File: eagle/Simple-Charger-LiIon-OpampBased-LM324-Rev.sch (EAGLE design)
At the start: 21 parts, among them IC1 LM324N, T1 BC327

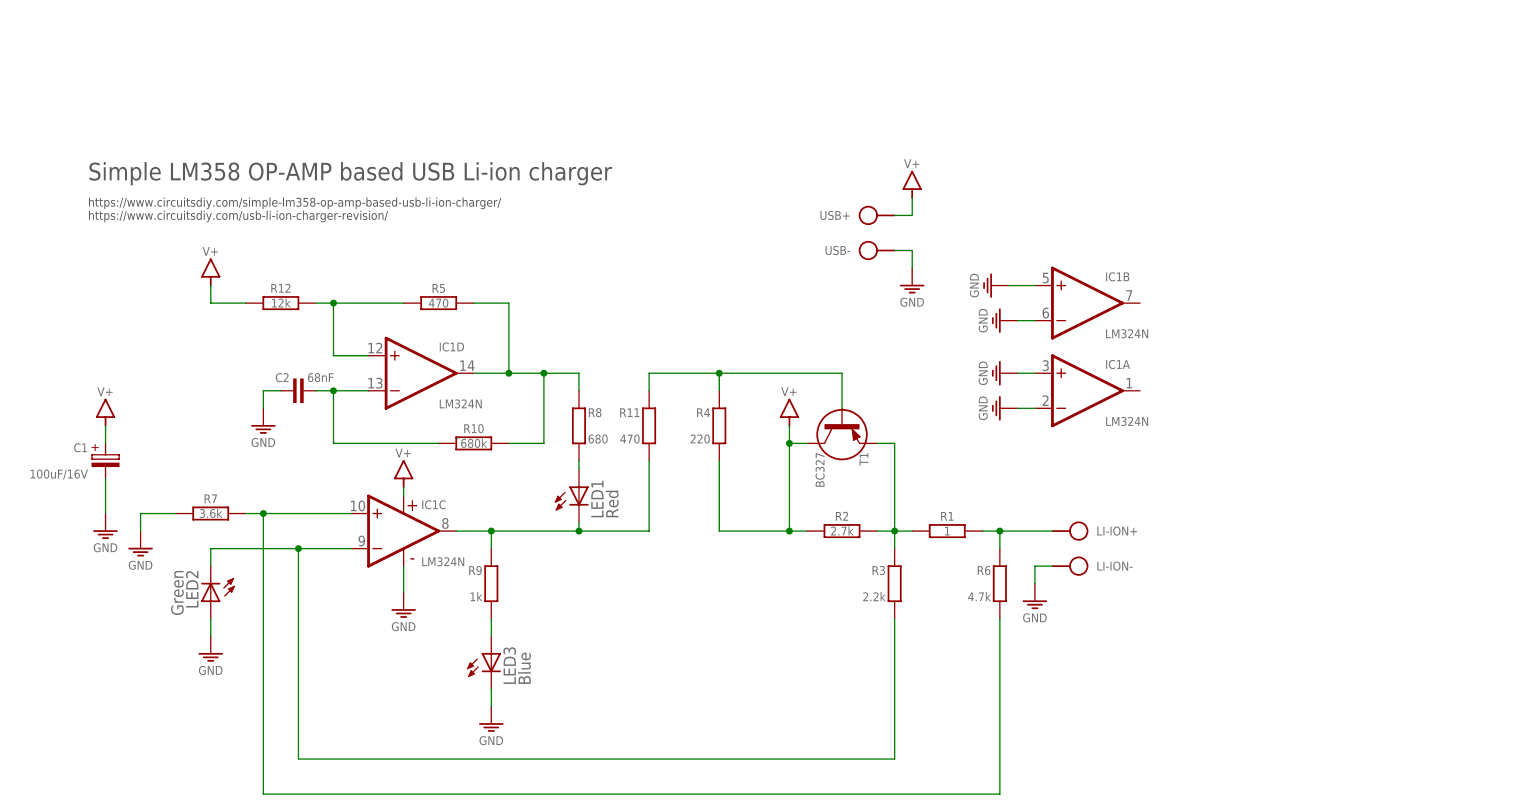
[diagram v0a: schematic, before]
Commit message: ...
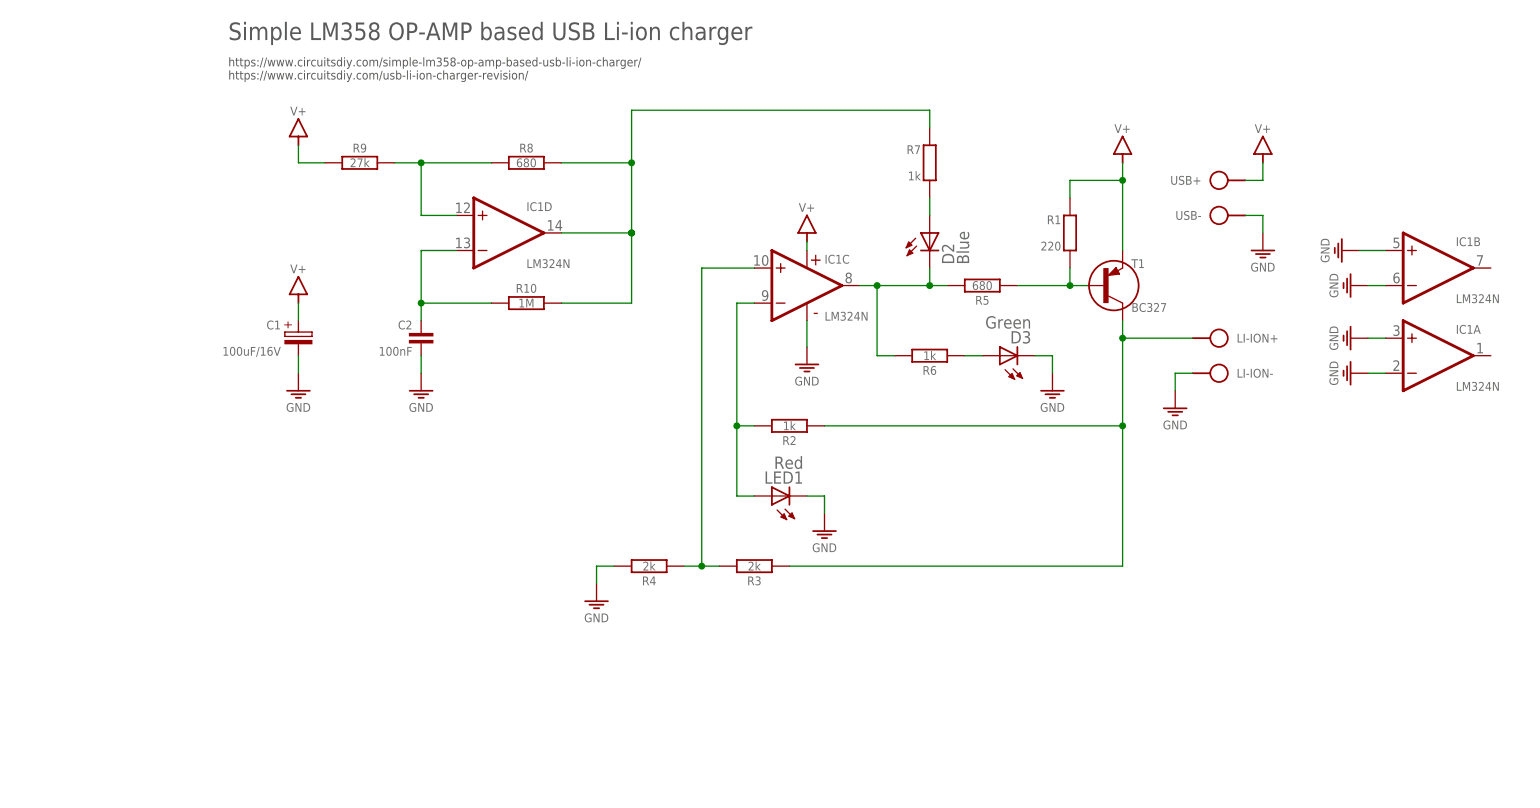
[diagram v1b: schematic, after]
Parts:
- removed LED2: Green, led:LED3MM
- removed LED3: Blue, led:LED3MM
- removed R11: 470, r:R0204/10-V
- removed R12: 12k, r:R-H0204/10-V
- added D2: Blue, led:LED3MM
- added D3: Green, led:LED3MM
- C2: value 68nF -> 100nF; device c:C-H050-020X044/V -> c:C050-020X044/V
- R1: value 1 -> 220; device r:R-H0204/10-V -> r:R0204/10-V
- R10: value 680k -> 1M; device r:R-H0204/2V -> r:R-H0204/10
- R2: value 2.7k -> 1k; device r:R-H0204/10-V -> r:R-H0204/10
- R3: value 2.2k -> 2k; device r:R0204/10-V -> r:R-H0204/10
- R4: value 220 -> 2k; device r:R0204/10 -> r:R-H0204/10
- R5: value 470 -> 680
- R6: value 4.7k -> 1k; device r:R0204/10-V -> r:R-H0204/10
- R7: value 3.6k -> 1k; device r:R-H0204/10-V -> r:R0204/10-V
- R8: device r:R0204/10 -> r:R-H0204/10
- R9: value 1k -> 27k; device r:R0204/10-V -> r:R-H0204/10-V
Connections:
- removed net N$12: LI-ION+.P$1, R1.2, R6.1
- removed net N$6: LED3.A, R9.2
- removed net N$9: R11.1, R4.1, T1.B
- new net N$10: LI-ION+.P$1, R2.1, R3.1, T1.C
- new net N$4: IC1D.OUT, R10.2, R7.1, R8.1
- net GND: now also C2.2, D3.C, LED1.C, R4.2; no longer C2.1, LED2.A, LED3.C, R7.1
- net N$1: now also R8.2, R9.2; no longer R12.2, R5.1
- net N$11: now also D3.A, R6.1; no longer R1.1, R2.2, R3.1, T1.E
- net N$13: now also R3.2, R4.1; no longer R6.2, R7.2
- net N$2: now also D2.A, R7.2; no longer IC1D.OUT, R10.2, R5.2, R8.1
- net N$3: now also C2.1; no longer C2.2
- net N$5: now also LED1.A, R2.2; no longer LED2.C, R3.2
- net N$7: now also D2.C, R5.2, R6.2; no longer LED1.C, R11.2, R9.1
- net N$8: now also R1.2, R5.1, T1.B; no longer LED1.A, R8.2
- net V+: now also R1.1, R9.1, T1.E; no longer R12.1, R2.1, R4.2, T1.C
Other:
- moved on the sheet: C1, IC1A, IC1B, IC1C, IC1D, LED1, LI-ION+, LI-ION-, R1, R10, R2, R3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

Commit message: ...
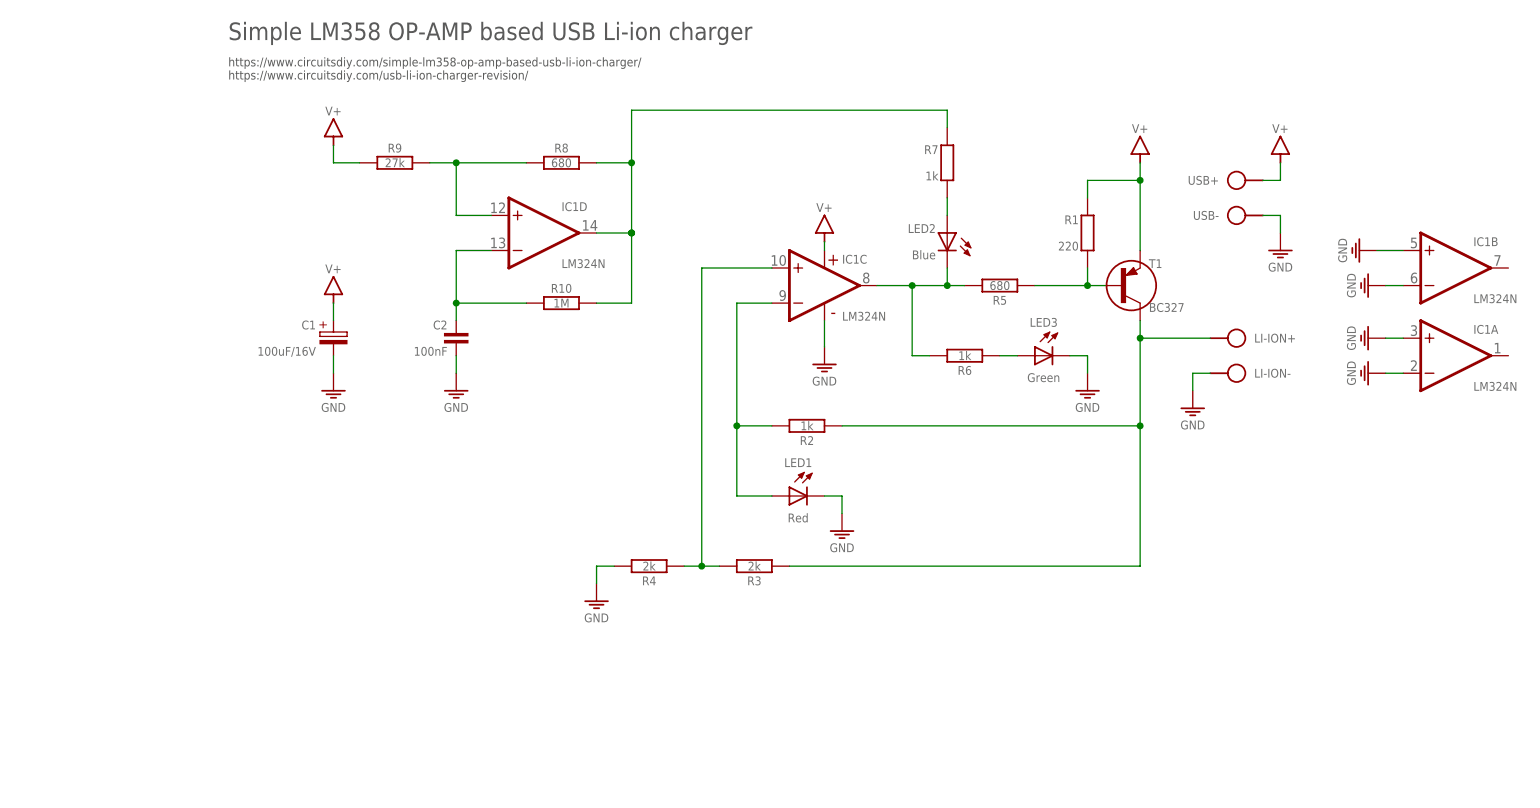
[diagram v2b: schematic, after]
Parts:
- removed D2: Blue, led:LED3MM
- removed D3: Green, led:LED3MM
- added LED2: Blue, d:LED-3MM
- added LED3: Green, d:LED-H-3MM
- C1: device c:CPOLE2,5-5/V -> c:CPOLE2.5-5
- LED1: device led:LED3MM -> d:LED-H-3MM
- R10: device r:R-H0204/10 -> r:R-H0204/2.54
- R4: device r:R-H0204/10 -> r:R-H0204/12-V
- R7: device r:R0204/10-V -> r:R0204/10
- R9: device r:R-H0204/10-V -> r:R-H0204/10
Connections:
- net GND: now also LED1.K, LED3.K; no longer D3.C, LED1.C
- net N$11: now also LED3.A; no longer D3.A
- net N$2: now also LED2.A; no longer D2.A
- net N$7: now also LED2.K; no longer D2.C
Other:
- moved on the sheet: C1, C2, IC1A, IC1B, IC1C, IC1D, LED1, LI-ION+, LI-ION-, R1, R10, R2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
